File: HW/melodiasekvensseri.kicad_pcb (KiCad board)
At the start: 2 copper layers, 60.6 x 110 mm, 58 parts, among them IC1 74LS138, J1 Conn_02x05_Odd_Even, J2 Clock_In, J3 Gate_Out, J4 CV_Out, J5 Conn_02x03_Odd_Even, J6 Conn_01x04, U1 TLV2372IP

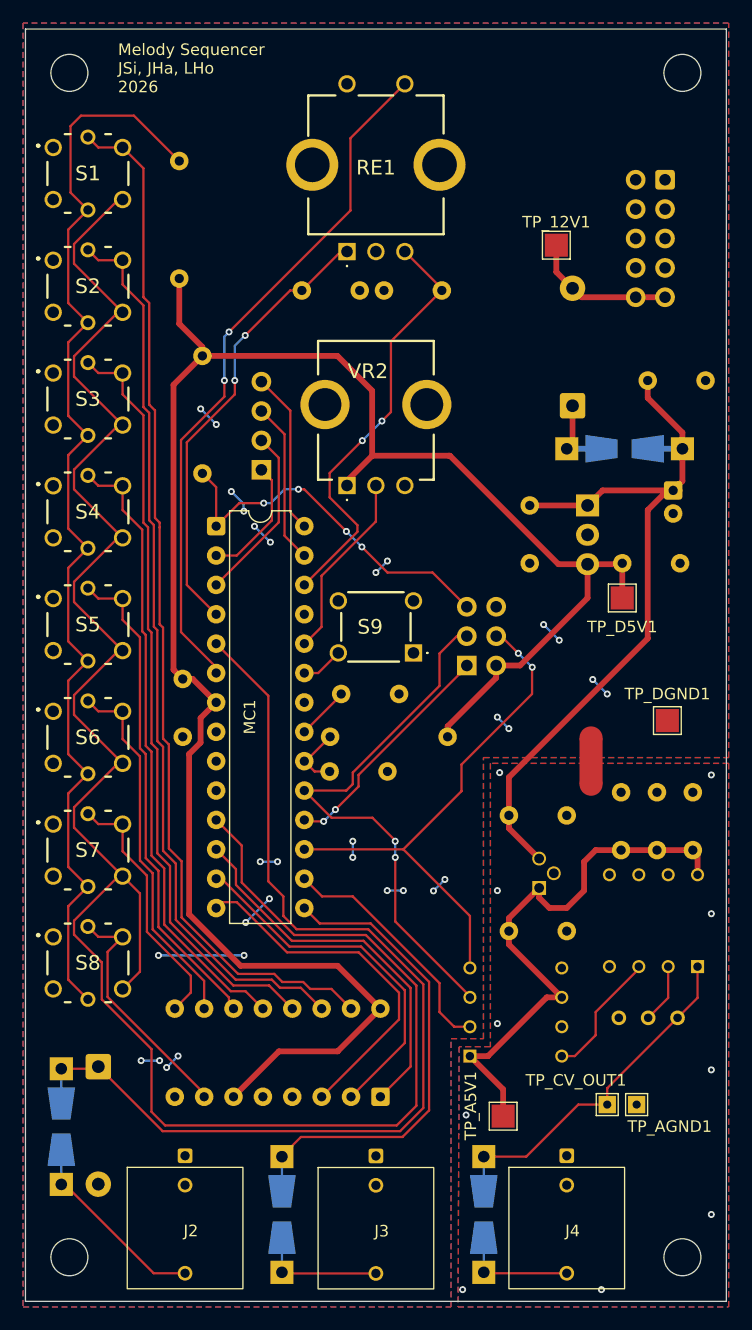
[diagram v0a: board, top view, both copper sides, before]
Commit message: Cleanup traces
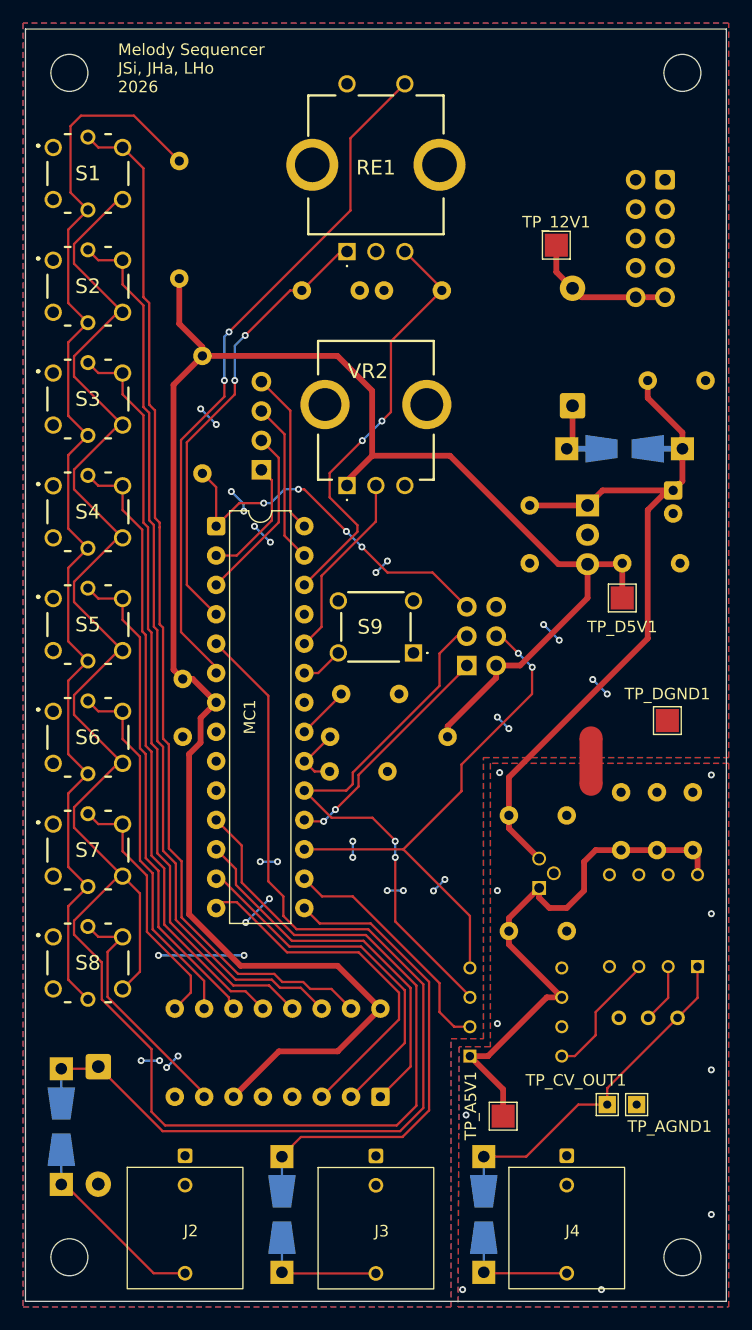
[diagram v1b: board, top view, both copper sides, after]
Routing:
- net +12V: track 66.7 -> 65.6 mm
- net ENC_B: track 37.8 -> 36.9 mm
- net Net-(MC1-AREF): track 4.74 -> 3.92 mm
- net Net-(D1-K): track 6.93 -> 6.22 mm
- net ENC_A: track 39.1 -> 38.5 mm
- net ENC_S: track 60.2 -> 59.7 mm
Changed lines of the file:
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@@
 		(capping no)
 		(filling no)
-		(zone_defaults)
 		(pcbplotparams
 			(layerselection 0x00000000_00000000_55555555_575555ff)
@@
 	(segment
 		(start 149.675 73.4)
-		(end 156.3 73.4)
-		(width 0.5)
-		(layer "F.Cu")
-		(net "D_+5V")
-	)
-	(segment
-		(start 171.22 82.78)
-		(end 171.3 82.7)
+		(end 156.4 73.4)
 		(width 0.5)
 		(layer "F.Cu")
@@
 	)
 	(segment
-		(start 156.4 73.4)
-		(end 156.3 73.4)
-		(width 0.5)
-		(layer "F.Cu")
-		(net "D_+5V")
-	)
-	(segment
 		(start 149.675 67.775)
 		(end 149.675 73.4)
@@
 	)
 	(segment
-		(start 143.81 89.65)
-		(end 143.85 89.65)
-		(width 0.2)
-		(layer "F.Cu")
-		(net "TEMPO")
-	)
-	(segment
 		(start 152.5 111)
 		(end 152.373789 111)
@@
 	)
 	(segment
-		(start 147.5 55.75)
-		(end 146.963132 55.75)
-		(width 0.2)
-		(layer "F.Cu")
-		(net "ENC_A")
-	)
-	(segment
 		(start 133.65 72.25)
 		(end 133.65 84.57)
@@
 	)
 	(segment
-		(start 155.7 58.95)
-		(end 155.7 59.113132)
-		(width 0.2)
-		(layer "F.Cu")
-		(net "ENC_B")
-	)
-	(segment
 		(start 152.5 55.75)
 		(end 155.7 58.95)
@@
 	)
 	(segment
-		(start 152.95 55.263132)
-		(end 152.2 55.263132)
-		(width 0.2)
-		(layer "F.Cu")
-		(net "ENC_B")
-	)
-	(segment
 		(start 143.81 84.57)
 		(end 148.4 79.98)
@@
 		(net "ENC_S")
 	)
-	(segment
-		(start 136.19 91.69)
-		(end 136.19 92.19)
-		(width 0.2)
-		(layer "F.Cu")
-		(net "ENC_S")
-	)
 	(via
 		(at 137.3 62.7)
@@
 	)
 	(segment
-		(start 125.82126 126.39874)
-		(end 126 126.22)
-		(width 0.2)
-		(layer "F.Cu")
-		(net "CLK_IN")
-	)
-	(segment
 		(start 143.146566 114.33946)
 		(end 142 113.192894)
@@
 	)
 	(segment
-		(start 143.84 110)
-		(end 143.81 109.97)
-		(width 0.2)
-		(layer "F.Cu")
-		(net "DAC_CS")
-	)
-	(segment
 		(start 155.5 119)
 		(end 148 111.5)
@@
 	)
 	(segment
-		(start 160.830469 89)
-		(end 160.4 89)
-		(width 0.2)
-		(layer "F.Cu")
-		(net "SPI_MOSI")
-	)
-	(segment
 		(start 163.5 91.702083)
 		(end 163.5 94)
@@
 	)
 	(segment
-		(start 143.934975 105.014975)
-		(end 143.81 104.89)
-		(width 0.2)
-		(layer "F.Cu")
-		(net "SPI_MISO")
-	)
-	(segment
 		(start 148.5 102)
 		(end 148.5 101)
@@
 	)
 	(segment
-		(start 157.86 91.64)
-		(end 157.86 91.54)
-		(width 0.2)
-		(layer "F.Cu")
-		(net "SPI_MISO")
-	)
-	(segment
 		(start 146.5 104)
 		(end 148.5 102)
@@
 	)
 	(segment
-		(start 158.13 120.23)
-		(end 158.13 120.13)
-		(width 0.2)
-		(layer "F.Cu")
-		(net "SPI_SCK")
-	)
-	(segment
 		(start 157 89)
 		(end 155.5 90.5)
@@
 	)
 	(segment
-		(start 143.93 99.81)
-		(end 143.81 99.81)
-		(width 0.2)
-		(layer "F.Cu")
-		(net "Net-(MC1-AVCC)")
-	)
-	(segment
-		(start 143.81 97.19)
-		(end 143.81 97.27)
-		(width 0.2)
-		(layer "F.Cu")
-		(net "Net-(MC1-AREF)")
-	)
-	(segment
-		(start 143.81 97.27)
-		(end 144.13 97.27)
-		(width 0.2)
-		(layer "F.Cu")
-		(net "Net-(MC1-AREF)")
-	)
-	(segment
-		(start 146.58 94.5)
-		(end 147 94.5)
-		(width 0.2)
-		(layer "F.Cu")
-		(net "Net-(MC1-AREF)")
-	)
-	(segment
 		(start 143.81 97.27)
 		(end 146.58 94.5)
@@
 	)
 	(segment
-		(start 122.8 136.093132)
-		(end 130.79 144.083132)
-		(width 0.2)
-		(layer "F.Cu")
-		(net "Net-(J2-PadT)")
-	)
-	(segment
-		(start 130.79 144.083132)
-		(end 133.5 144.083132)
-		(width 0.2)
-		(layer "F.Cu")
-		(net "Net-(J2-PadT)")
-	)
-	(segment
-		(start 122.8 133.39898)
-		(end 122.8 136.40126)
-		(width 0.2)
-		(layer "B.Cu")
-		(net "Net-(J2-PadT)")
-	)
-	(segment
 		(start 167.5 129.5)
 		(end 163.00126 133.99874)
@@
 	)
 	(segment
+		(start 122.8 136.093132)
+		(end 130.79 144.083132)
+		(width 0.2)
+		(layer "F.Cu")
+		(net "Net-(J2-PadT)")
+	)
+	(segment
+		(start 130.79 144.083132)
+		(end 133.5 144.083132)
+		(width 0.2)
+		(layer "F.Cu")
+		(net "Net-(J2-PadT)")
+	)
+	(segment
+		(start 122.8 133.39898)
+		(end 122.8 136.40126)
+		(width 0.2)
+		(layer "B.Cu")
+		(net "Net-(J2-PadT)")
+	)
+	(segment
 		(start 137.296026 120.243689)
 		(end 137.296026 121.203132)
@@
 	)
 	(segment
-		(start 175.7 76.4)
-		(end 176.3 76.4)
-		(width 0.5)
-		(layer "F.Cu")
-		(net "+12V")
-	)
-	(segment
 		(start 173.5 78.1)
 		(end 173.5 89.2)
@@
 	)
 	(segment
-		(start 175.7 76.4)
-		(end 175.2 76.4)
-		(width 0.5)
-		(layer "F.Cu")
-		(net "+12V")
-	)
-	(segment
 		(start 173.5 66.9)
 		(end 173.5 68.4)
@@
 	)
 	(segment
-		(start 172.73 117.77)
-		(end 172.73 117.57)
-		(width 0.2)
-		(layer "F.Cu")
-		(net "Net-(DAC1-VOUT)")
-	)
-	(segment
 		(start 169 123.5)
 		(end 169 121.5)
@@
 	)
 	(segment
-		(start 167 72.29874)
-		(end 166.49874 72.8)
-		(width 0.5)
-		(layer "F.Cu")
-		(net "Net-(D1-K)")
-	)
-	(segment
